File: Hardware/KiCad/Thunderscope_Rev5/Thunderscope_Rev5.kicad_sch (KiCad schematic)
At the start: 12 parts

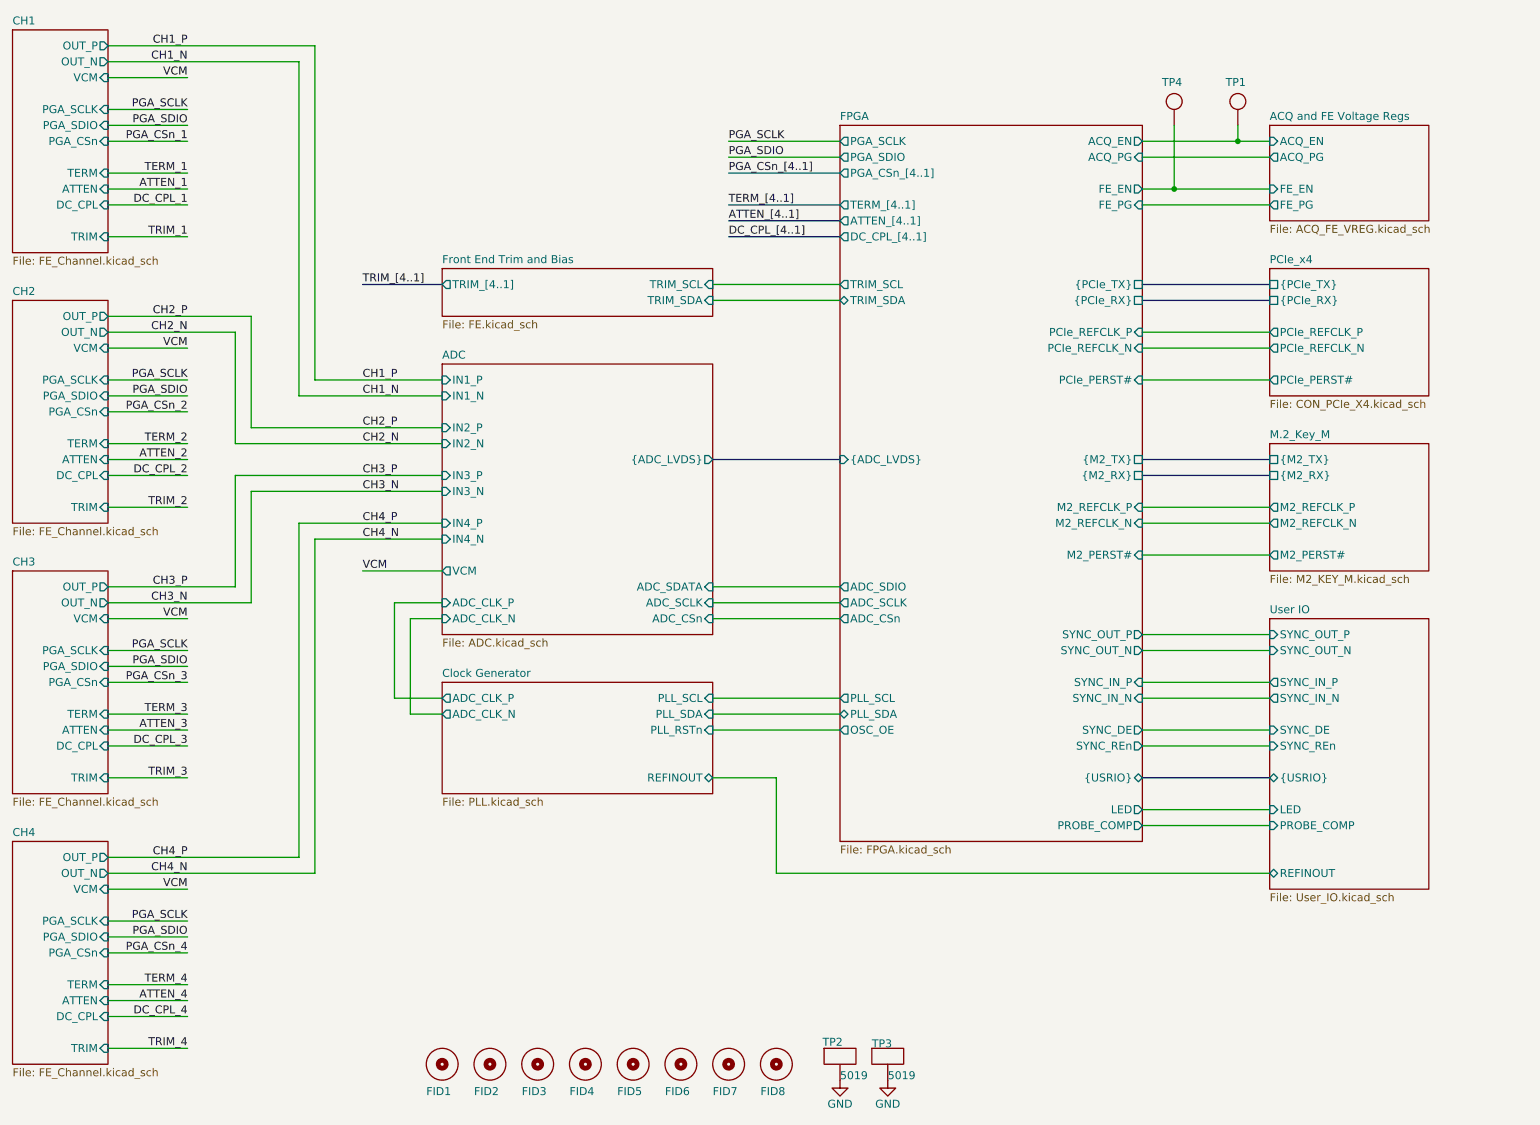
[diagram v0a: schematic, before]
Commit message: Schematic cleanup and RGB status LED
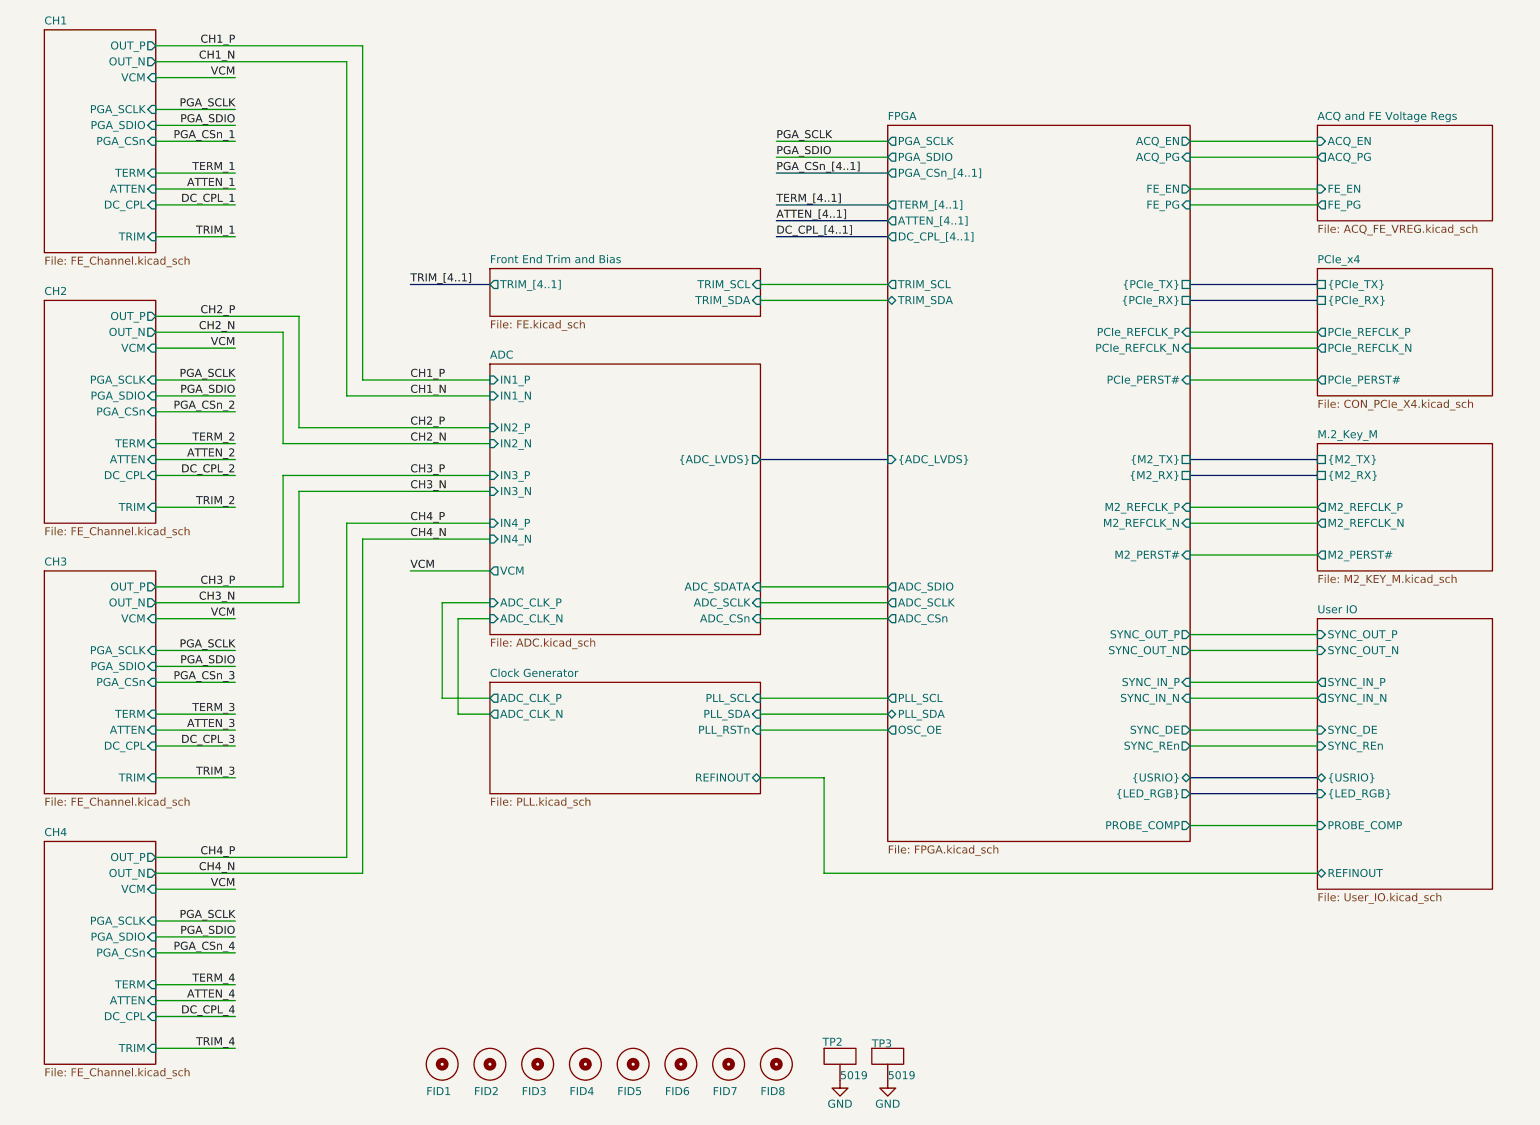
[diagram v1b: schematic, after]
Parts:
- removed TP1, TP4: PCB, Thunderscope_Rev5:GEN_TP_PCB, symbol Thunderscope_Rev5:TP PCB 1mm
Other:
- sheet FPGA ports: added {LED_RGB}; removed LED
- sheet User IO ports: added {LED_RGB}; removed LED
